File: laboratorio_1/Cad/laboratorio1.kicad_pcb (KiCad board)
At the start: 2 copper layers, 31 parts, among them J5 Output, U1 TL084, U2 TL084, j1 Vdd, j2 Vss, j3 GND, j4 Input

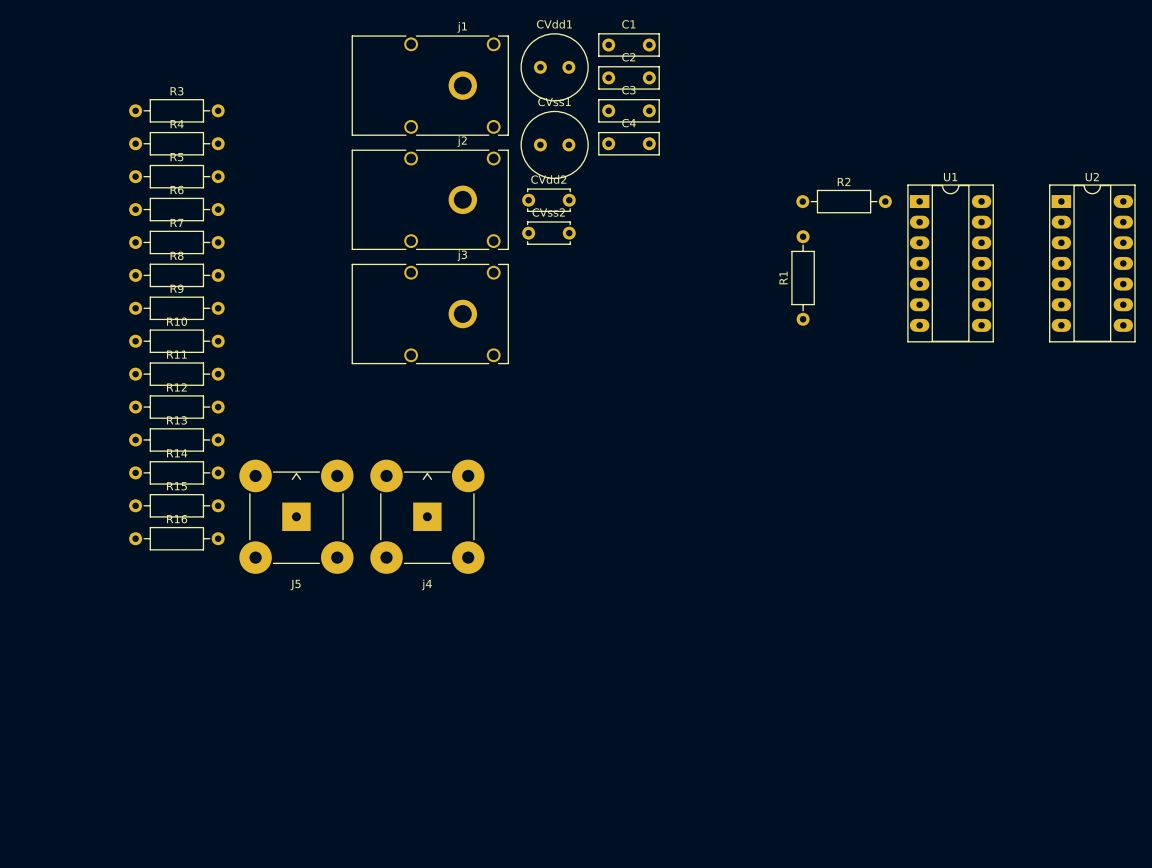
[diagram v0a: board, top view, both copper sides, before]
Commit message: ahora si actualizo con windows el kicad
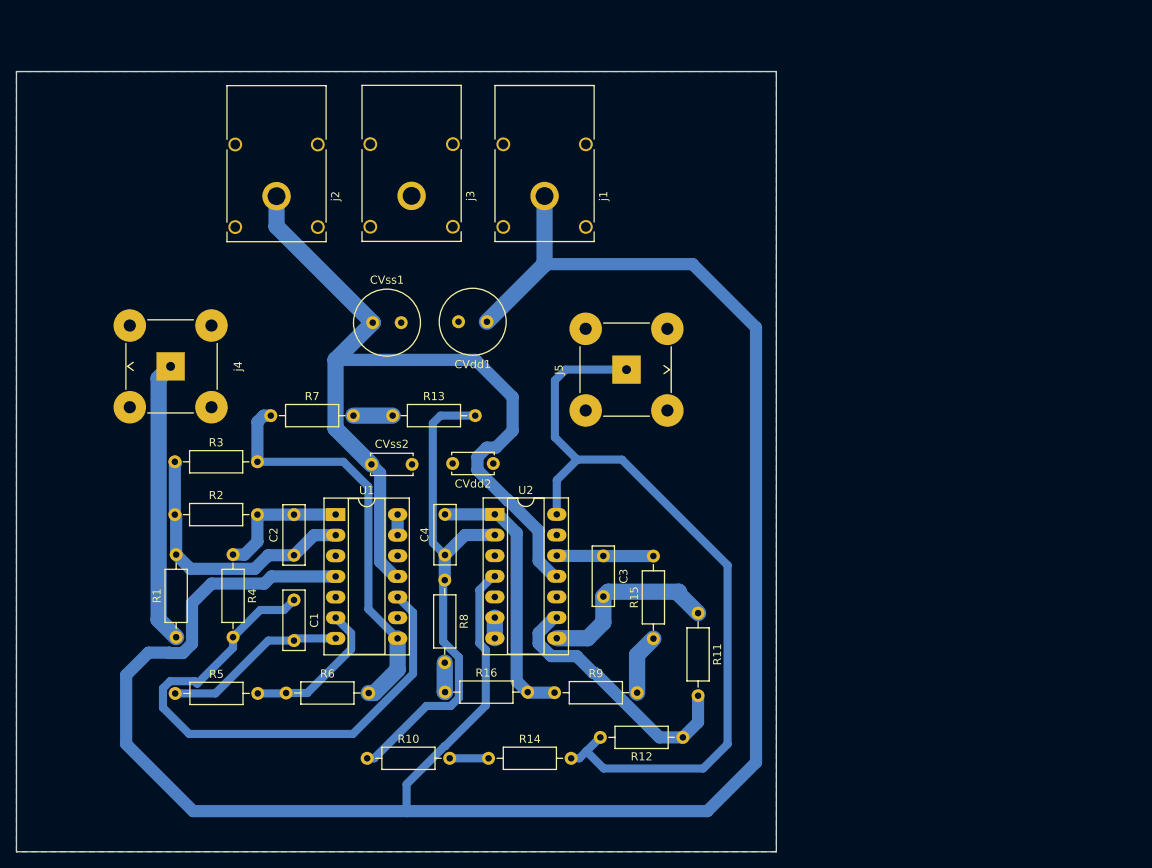
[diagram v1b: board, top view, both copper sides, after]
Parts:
- R11, R12: value R -> 1k
- moved R1 86.5 mm to (115.7, 125.1)
- moved R2 86.3 mm to (115.5, 110.0)
- moved U1 81.5 mm to (135.3, 110.0)
- moved U2 79.6 mm to (154.9, 110.0)
- moved R12 78.7 mm to (178.0, 137.4), turned to 180 degrees
- moved C1 78.5 mm to (130.2, 120.5), turned to -90 degrees
- moved R11 75.2 mm to (179.9, 122.1), turned to -90 degrees
- moved C2 70.3 mm to (130.2, 115.0), turned to 90 degrees
- moved R9 70.0 mm to (162.2, 131.9)
- moved R15 65.8 mm to (174.4, 125.3), turned to 90 degrees
- moved R5 63.8 mm to (115.5, 132.0)
- moved R6 62.3 mm to (129.2, 132.0)
- moved R10 58.7 mm to (139.2, 140.0)
- moved R14 55.9 mm to (154.1, 140.0)
- moved C3 54.8 mm to (168.2, 115.1), turned to -90 degrees
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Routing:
- net Net-(U1E-V+): track 0.00 -> 261.0 mm
- net Net-(U1E-V-): track 0.00 -> 109.4 mm
- net Net-(J5-In): track 0.00 -> 98.1 mm
- net Net-(U1C-+): track 0.00 -> 69.8 mm
- net Net-(U2A--): track 0.00 -> 62.4 mm
- net Net-(R3-Pad2): track 0.00 -> 50.6 mm
- net Net-(j4-In): track 0.00 -> 34.8 mm
- net Net-(U1A--): track 0.00 -> 33.8 mm
- net Net-(C4-Pad2): track 0.00 -> 33.2 mm
- net Net-(U2C--): track 0.00 -> 32.7 mm
- net Net-(C3-Pad2): track 0.00 -> 22.9 mm
- net Net-(C1-Pad2): track 0.00 -> 22.6 mm
- net Net-(U1B--): track 0.00 -> 18.4 mm
- net Net-(C2-Pad2): track 0.00 -> 16.6 mm
- net Net-(U2D-+): track 0.00 -> 11.9 mm
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- added copper zone on B.Cu, net GND
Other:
- board outline added: 93.5 x 96 mm
- board text added: "R5"
